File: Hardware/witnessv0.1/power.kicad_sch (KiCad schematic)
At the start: 2 parts, among them U2 XL1509-3.3, U3 MC33063AD

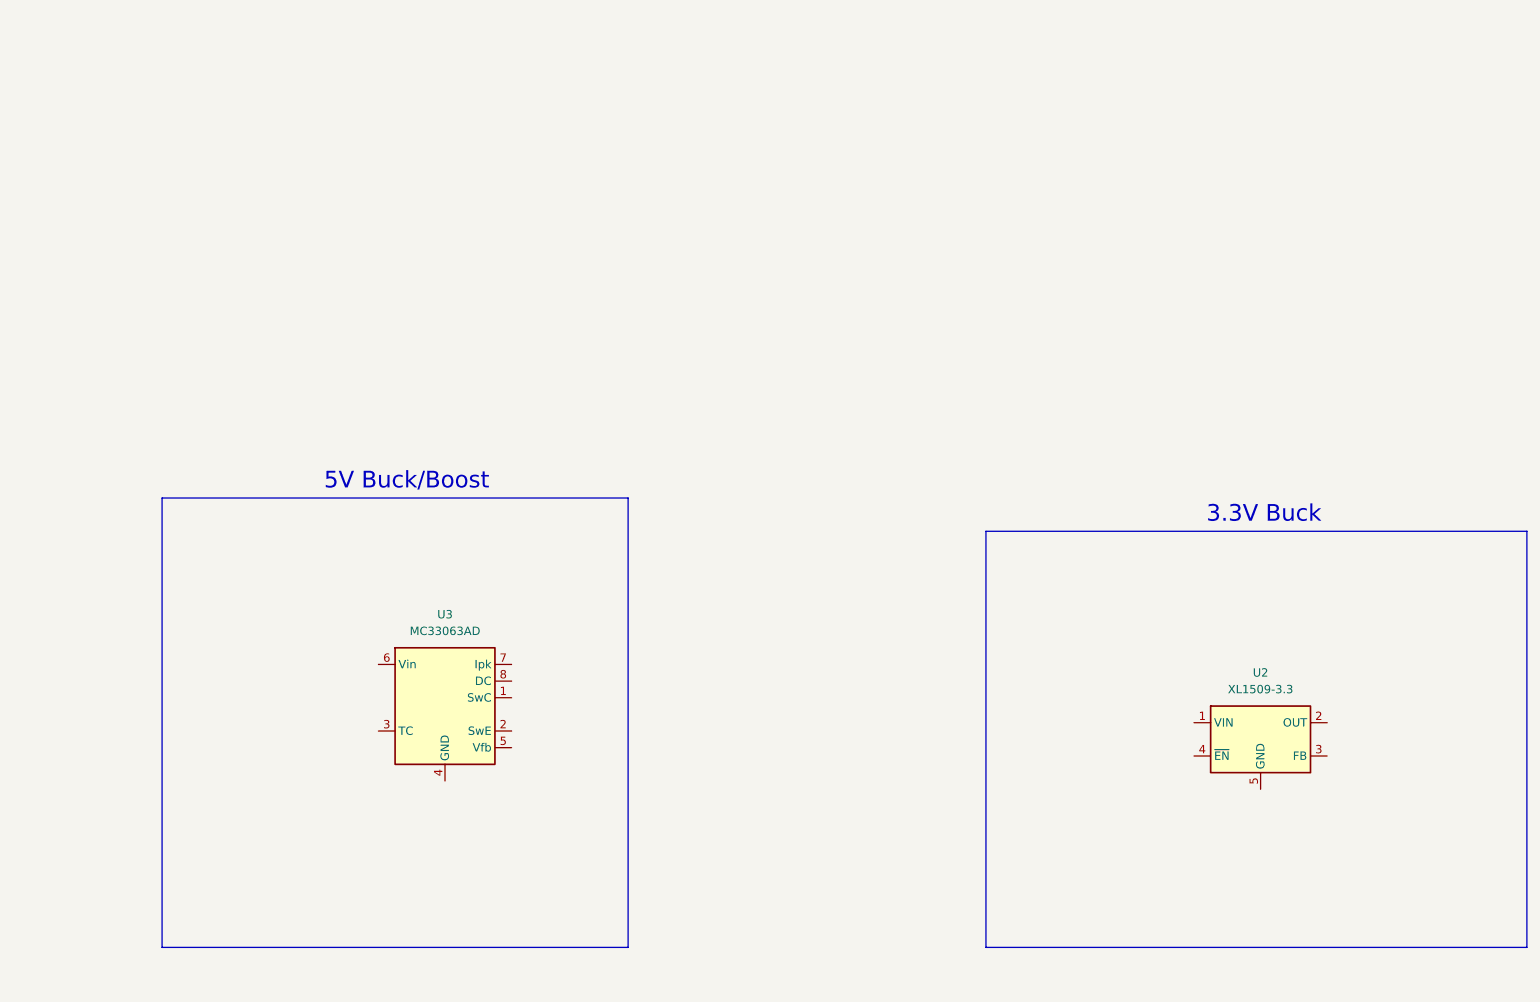
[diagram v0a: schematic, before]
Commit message: power updates and some esp32 stuff
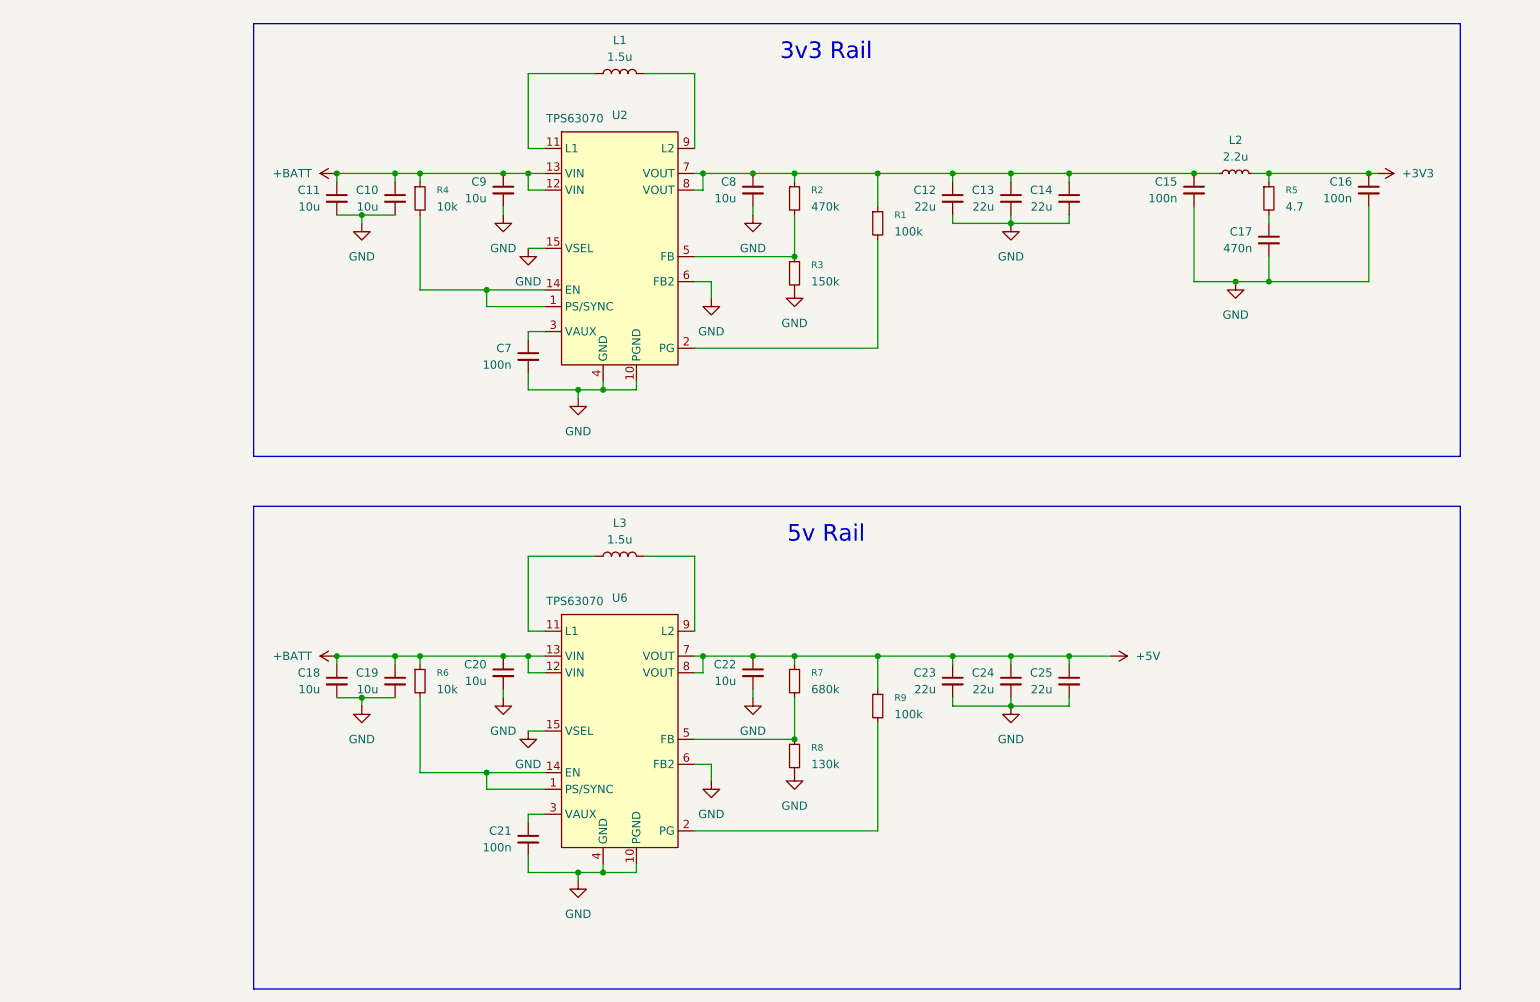
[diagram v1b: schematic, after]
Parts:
- removed U2: XL1509-3.3, Package_SO:SOIC-8_3.9x4.9mm_P1.27mm, symbol Regulator_Switching:XL1509-3.3
- removed U3: MC33063AD, Package_SO:SOIC-8_3.9x4.9mm_P1.27mm, symbol Regulator_Switching:MC33063AD
- added C10, C11, C18, C19: 10u, Capacitor_SMD:C_0805_2012Metric, symbol Device:C_Small
- added C12, C13, C14, C23, C24, C25: 22u, Capacitor_SMD:C_0805_2012Metric, symbol Device:C_Small
- added C15, C16, C21, C7: 100n, Capacitor_SMD:C_0603_1608Metric, symbol Device:C_Small
- added C17: 470n, Capacitor_SMD:C_0603_1608Metric, symbol Device:C_Small
- added C20, C22, C8, C9: 10u, Capacitor_SMD:C_0603_1608Metric, symbol Device:C_Small
- added L1, L3: 1.5u, Inductor_SMD:L_1210_3225Metric, symbol Device:L
- added L2: 2.2u, Inductor_SMD:L_1206_3216Metric, symbol Device:L_Small
- added R1, R9: 100k, Resistor_SMD:R_0603_1608Metric, symbol Device:R_Small
- added R2: 470k, Resistor_SMD:R_0603_1608Metric, symbol Device:R_Small
- added R3: 150k, Resistor_SMD:R_0603_1608Metric, symbol Device:R_Small
- added R4, R6: 10k, Resistor_SMD:R_0603_1608Metric, symbol Device:R_Small
- added R5: 4.7, Resistor_SMD:R_0603_1608Metric, symbol Device:R_Small
- added R7: 680k, Resistor_SMD:R_0603_1608Metric, symbol Device:R_Small
- added R8: 130k, Resistor_SMD:R_0603_1608Metric, symbol Device:R_Small
- added U2, U6: TPS63070, Witness:RNM0015A, symbol Witness:TPS63070
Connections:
- new net: R7.2, R8.1, U6.5 (FB)
- new net: C12.1, C13.1, C14.1, C15.1, C8.1, L2.1, R1.1, R2.1, U2.7 (VOUT), U2.8 (VOUT)
- new net: R6.2, U6.1 (PS/SYNC), U6.14 (EN)
- new net: C17.1, R5.2
- new net: L3.1, U6.11 (L1)
- new net: L3.2, U6.9 (L2)
- new net: R1.2, U2.2 (PG)
- new net: R9.2, U6.2 (PG)
- new net: C21.1, U6.3 (VAUX)
- new net: C7.1, U2.3 (VAUX)
- new net: R4.2, U2.1 (PS/SYNC), U2.14 (EN)
- new net: L1.1, U2.11 (L1)
- new net: R2.2, R3.1, U2.5 (FB)
- new net: L1.2, U2.9 (L2)
- new net +3V3: C16.1, L2.2, R5.1
- new net +5V: C22.1, C23.1, C24.1, C25.1, R7.1, R9.1, U6.7 (VOUT), U6.8 (VOUT)
- new net +BATT: C10.1, C11.1, C18.1, C19.1, C20.1, C9.1, R4.1, R6.1, U2.12 (VIN), U2.13 (VIN), U6.12 (VIN), U6.13 (VIN)
- new net GND: C10.2, C11.2, C12.2, C13.2, C14.2, C15.2, C16.2, C17.2, C18.2, C19.2, C20.2, C21.2, C22.2, C23.2, C24.2, C25.2, C7.2, C8.2, C9.2, R3.2, R8.2, U2.10 (PGND), U2.15 (VSEL), U2.4 (GND), U2.6 (FB2), U6.10 (PGND), U6.15 (VSEL), U6.4 (GND), U6.6 (FB2)
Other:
- note added: "3v3 Rail"
- note added: "5v Rail"
- note removed: "3.3V Buck"
- note removed: "5V Buck/Boost"

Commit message: mcu work
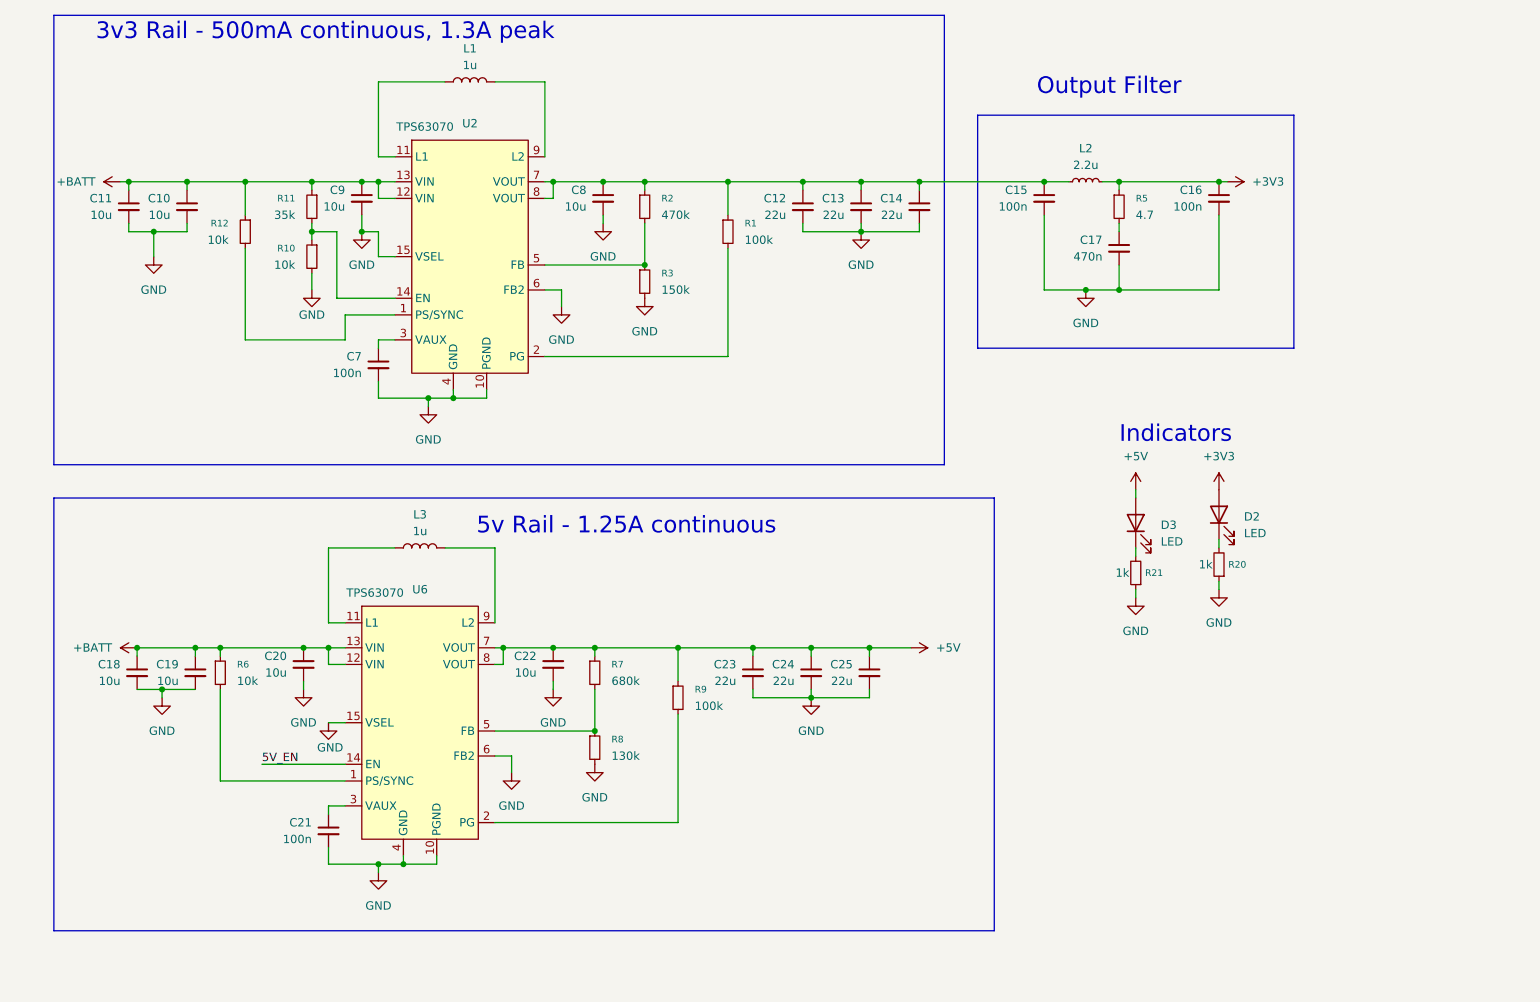
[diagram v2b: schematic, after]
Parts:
- removed R4: 10k, Resistor_SMD:R_0603_1608Metric, symbol Device:R_Small
- added D2, D3: LED, symbol Device:LED
- added R10, R12: 10k, Resistor_SMD:R_0603_1608Metric, symbol Device:R_Small
- added R11: 35k, Resistor_SMD:R_0603_1608Metric, symbol Device:R_Small
- added R20, R21: 1k, Resistor_SMD:R_0603_1608Metric, symbol Device:R_Small
- L1, L3: value 1.5u -> 1u
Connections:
- net +3V3: now also D2.2 (A)
- net +5V: now also D3.2 (A)
- net +BATT: now also R11.1, R12.1
- net GND: now also R10.2, R20.1, R21.1
- net at R6.2, U6.1 (PS/SYNC): no longer U6.14 (EN)
- net at U2.1 (PS/SYNC): now also R12.2; no longer U2.14 (EN)
- new net: D2.1 (K), R20.2
- new net: R10.1, R11.2, U2.14 (EN)
- new net: D3.1 (K), R21.2
- new net 5V_EN: U6.14 (EN)
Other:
- note added: "3v3 Rail - 500mA continuous, 1.3A peak"
- note added: "5v Rail - 1.25A continuous"
- note added: "Indicators"
- note added: "Output Filter"
- note removed: "3v3 Rail"
- note removed: "5v Rail"
- title: (none) -> Power
- moved on the sheet: C10, C11, C12, C13, C14, C15, C16, C17, C18, C19, C20, C21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
